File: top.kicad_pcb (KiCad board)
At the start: 2 copper layers, 85 parts, among them IC1 REG113NA-2.5_3K, IC2 LD39015M10R, J1 Conn_01x01_Male, J2 Conn_01x07_Male, SW1 SW_SPDT, U1 digital clock, U2 BC2AAPC, Y1 Crystal 32.768kHz

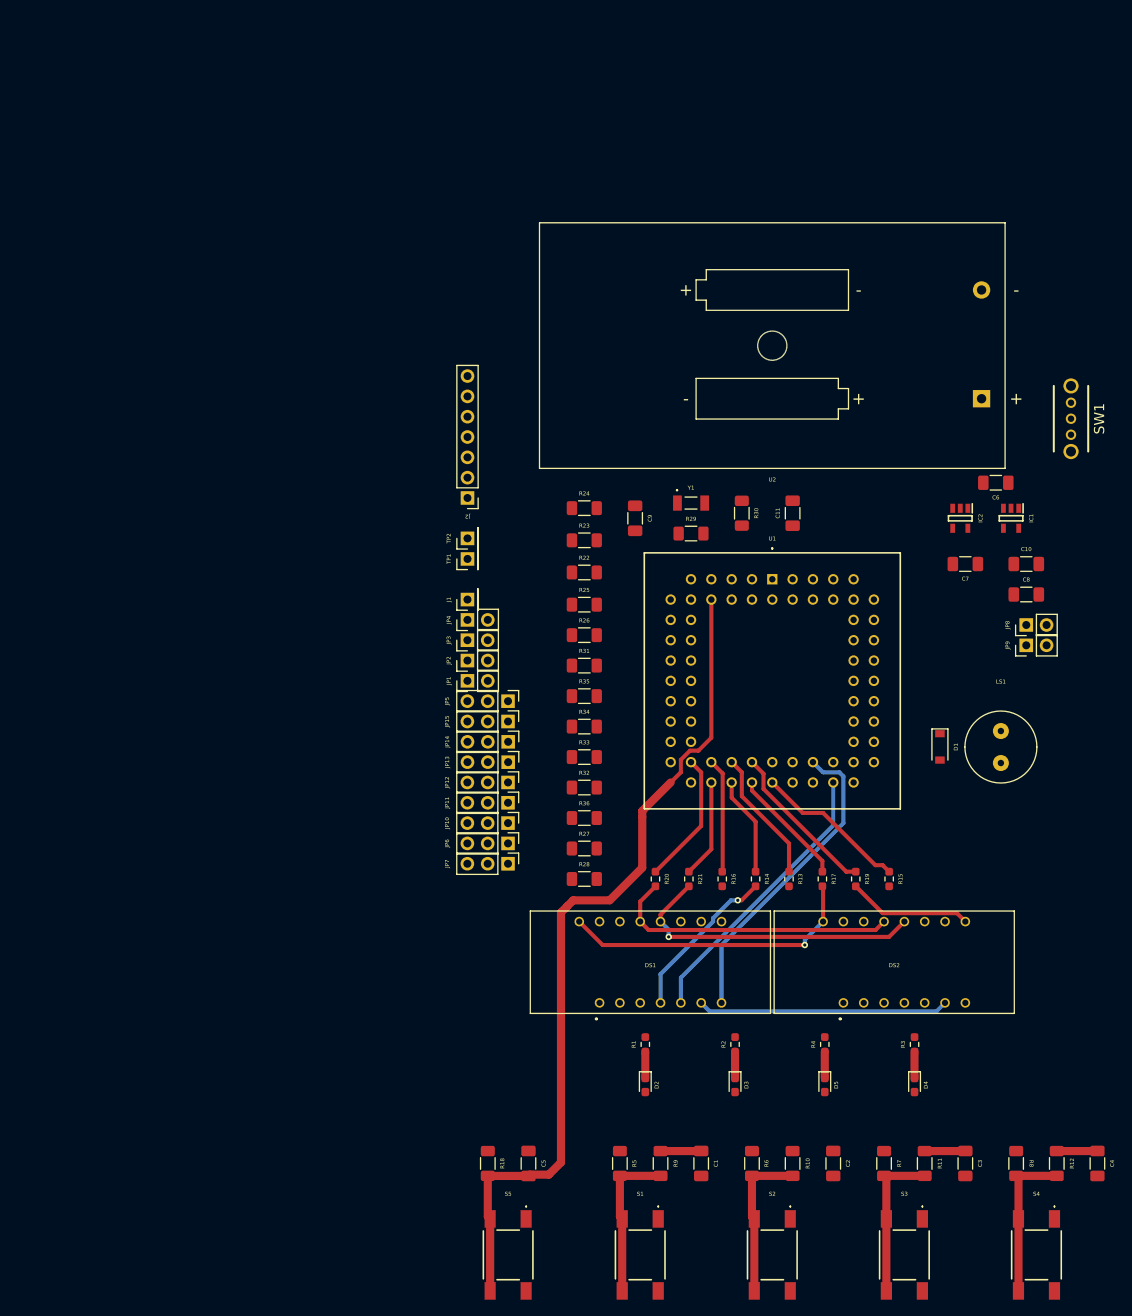
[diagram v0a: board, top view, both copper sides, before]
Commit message: Final
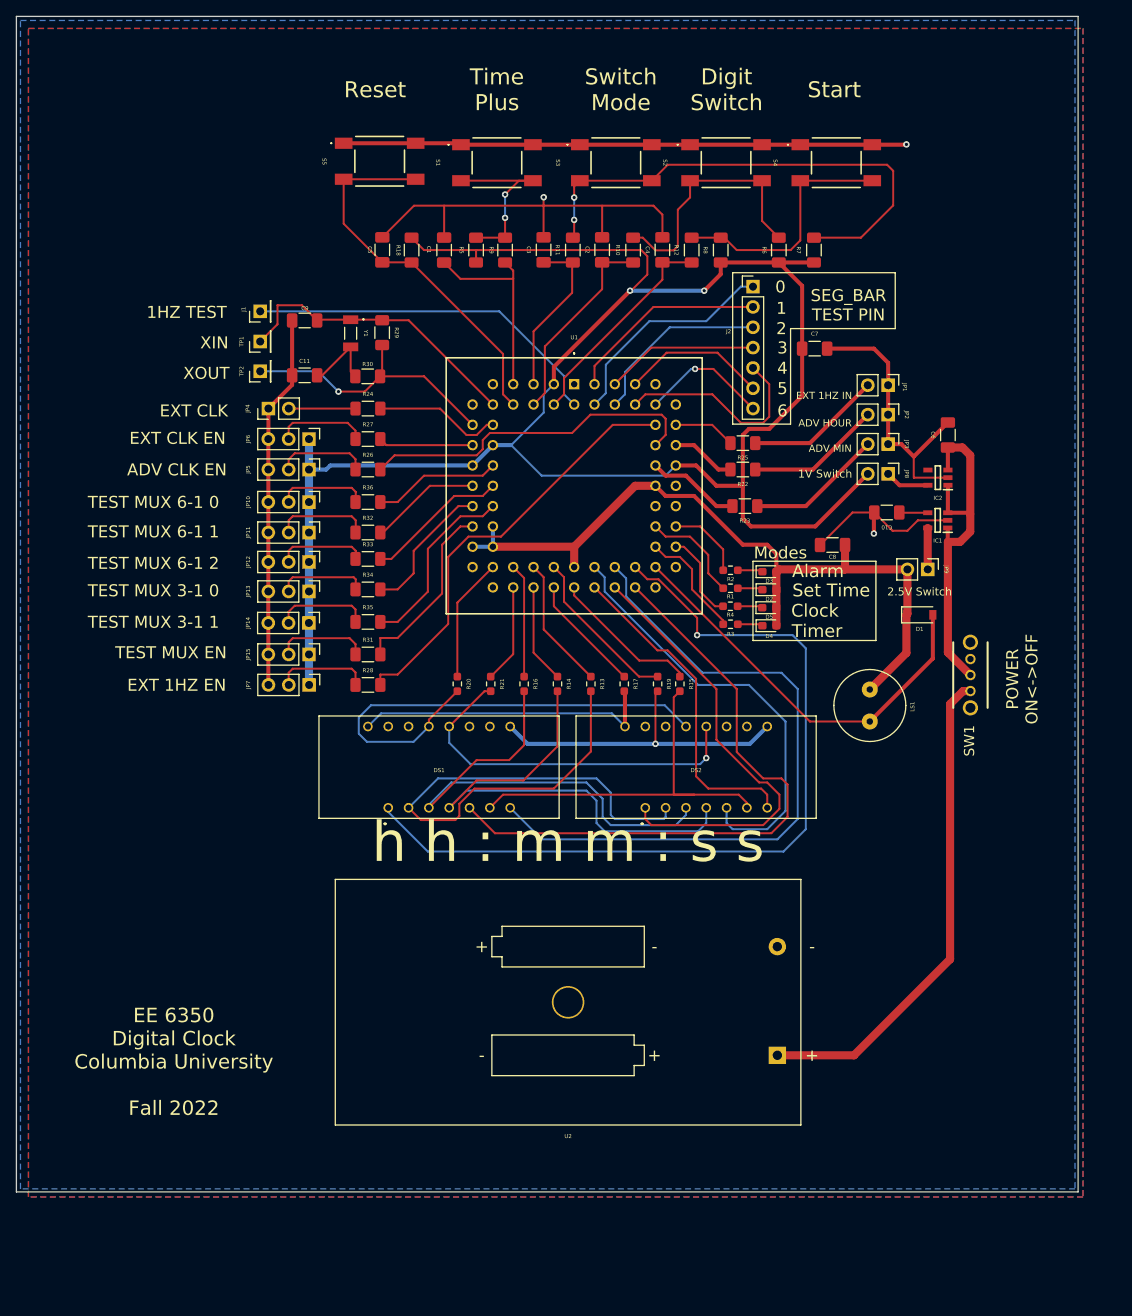
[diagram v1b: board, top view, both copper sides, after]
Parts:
- moved S3 141.2 mm to (117.6, 36.8), turned to 90 degrees
- moved S4 138.8 mm to (145.2, 36.8), turned to 90 degrees
- moved S1 137.7 mm to (102.7, 36.8), turned to 90 degrees
- moved S5 137.6 mm to (88.1, 36.6), turned to 90 degrees
- moved S2 136.6 mm to (131.4, 36.8), turned to 90 degrees
- moved C4 126.5 mm to (123.4, 47.7), turned to 90 degrees
- moved C3 125.8 mm to (108.6, 47.7), turned to 90 degrees
- moved R12 123.0 mm to (127.1, 47.8), turned to -90 degrees
- moved R11 122.4 mm to (112.2, 47.8), turned to -90 degrees
- moved R8 120.0 mm to (130.7, 47.8), turned to 90 degrees
- moved C1 118.6 mm to (96.1, 47.7), turned to 90 degrees
- moved C2 117.8 mm to (115.9, 47.7), turned to 90 degrees
- moved R10 115.9 mm to (119.8, 47.8), turned to -90 degrees
- moved R9 115.8 mm to (103.8, 47.8), turned to -90 degrees
- moved C5 115.7 mm to (88.4, 47.7)
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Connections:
- SW1 pad 4: (no net) -> GND
- SW1 pad 5: (no net) -> GND
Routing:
- net +1V0: track 0.00 -> 234.7 mm, vias 0 -> 2
- net GND: track 0.00 -> 227.6 mm, vias 0 -> 3
- net DIGIT_5: track 0.00 -> 105.3 mm, vias 0 -> 1
- net +2V5: track 0.00 -> 95.3 mm
- net Net-(DS1-Pad2): track 0.00 -> 74.1 mm
- net Net-(SW1-Pad3): track 0.00 -> 61.7 mm
- net Net-(DS1-Pad3): track 0.00 -> 60.5 mm
- net RESETN: track 106.2 -> 48.1 mm
- net DIGIT_2: track 0.00 -> 56.1 mm
- net DIGIT_1: track 0.00 -> 54.6 mm
- net EXTERNAL_1HZ_ENABLE: track 0.00 -> 53.5 mm
- net BUZZER: track 0.00 -> 51.4 mm
- net DIGIT_3: track 39.2 -> 85.4 mm
- net ONE_HZ_TEST: track 0.00 -> 45.4 mm
- net +3V0: track 0.00 -> 44.8 mm
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- added copper zone on B.Cu, net GND
- added copper zone on F.Cu, net GND
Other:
- board outline added: 132.7 x 146.9 mm
- board text added: "0"
- board text added: "1"
- board text added: "1HZ TEST"
- board text added: "1V Switch"
- board text added: "2"
- board text added: "2.5V Switch"
- board text added: "3"
- board text added: "4"
- board text added: "5"
- board text added: "6"
- board text added: "ADV CLK EN"
- board text added: "ADV HOUR"
- board text added: "ADV MIN"
- board text added: "Alarm"
- board text added: "Clock"
- board text added: "Digit Switch"
- board text added: "EE 6350 Digital Clock Columbia University Fall 2022"
- board text added: "EXT 1HZ EN"
- board text added: "EXT 1HZ IN"
- board text added: "EXT CLK"
- board text added: "EXT CLK EN"
- board text added: "Modes"
- board text added: "POWER ON<->OFF"
- board text added: "Reset"
- board text added: "SEG_BAR TEST PIN"
- board text added: "Set Time"
- board text added: "Start"
- board text added: "Switch Mode"
- board text added: "TEST MUX 3-1 0"
- board text added: "TEST MUX 3-1 1"
- board text added: "TEST MUX 6-1 0"
- board text added: "TEST MUX 6-1 1"
- board text added: "TEST MUX 6-1 2"
- board text added: "TEST MUX EN"
- board text added: "Time Plus"
- board text added: "Timer"
- board text added: "XIN"
- board text added: "XOUT"
- board text added: "h h : m m : s s"
